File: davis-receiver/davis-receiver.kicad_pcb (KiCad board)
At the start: 4 copper layers, 127 x 88.9 mm, 150 parts, among them J1 Conn_Coaxial, J2 Wurth_74982104400, J3 JTAG, J4 UART, J5 SPI-BARO, J6 SPI-RF, Q1 FDC2512, SW1 MCU_RESET, T1 POE70P-33, U1 TM4C129ENCZADI3R, U2 CC1125RHBR, U3 FXPS7115D4, U4 TPS79930DDCR, U5 MB10S, U6 MB10S, U7 TPS23753A, U8 FOD817A3SD, U9 TLV431ACDBZR, X1 ECS-2520MV-400-AY-TR, Y1 LFXTAL071758CUTT

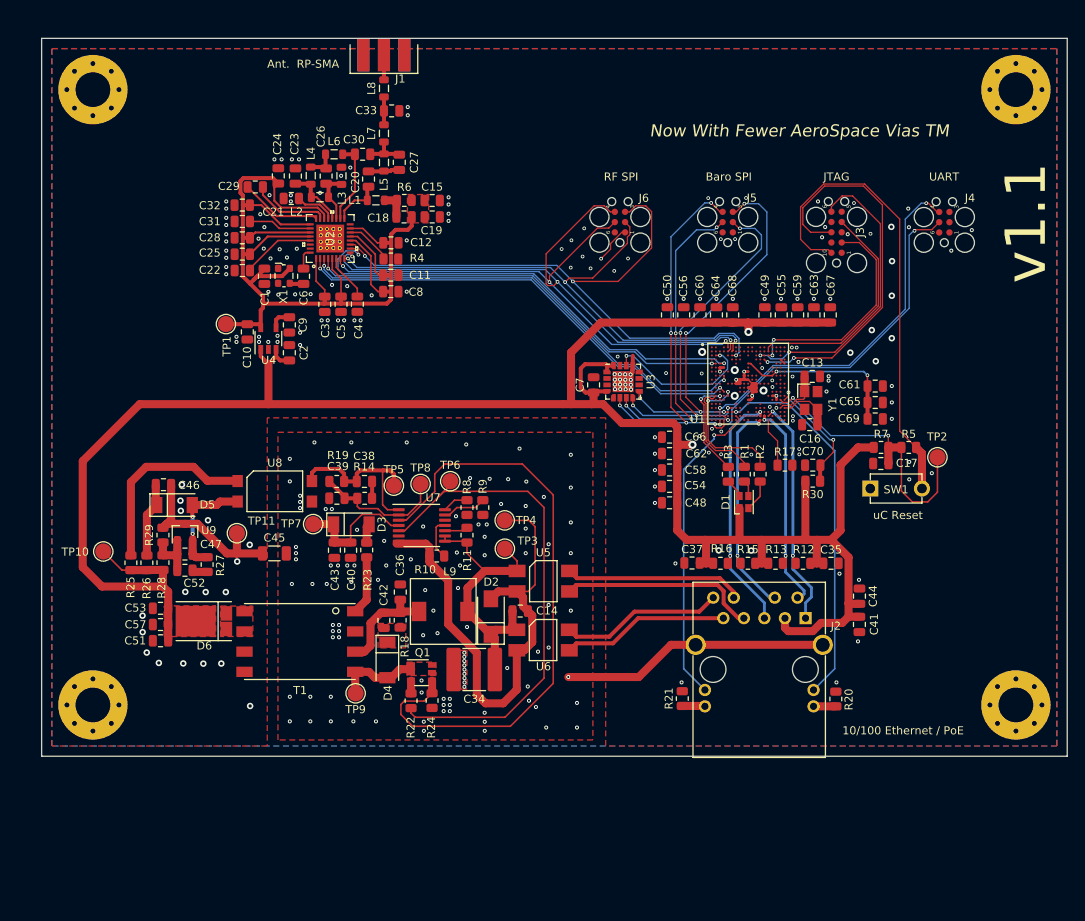
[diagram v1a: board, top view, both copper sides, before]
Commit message: Updates to DavisReceiver
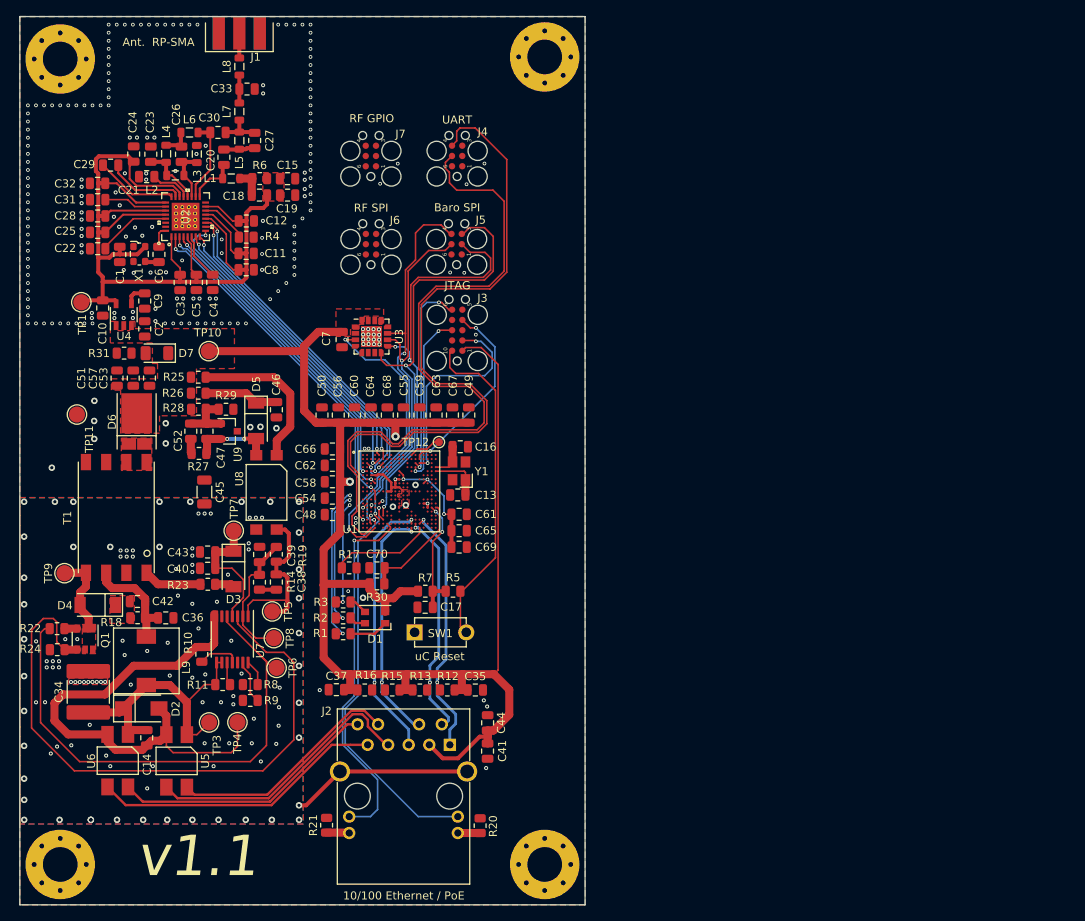
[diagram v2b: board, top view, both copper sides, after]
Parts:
- removed TP2: TestPoint, TestPoint:TestPoint_Pad_D2.0mm
- added D7: LED, LED_SMD:LED_1206_3216Metric, F.Cu at (39.0, 63.7)
- added J7: GPIO-RF, Custom:TC2030-IDC-FP, F.Cu at (65.5, 39.3)
- added R31: 100, Resistor_SMD:R_0805_2012Metric, F.Cu at (34.9, 63.7)
- added TP12: TestPoint, TestPoint:TestPoint_Pad_D1.0mm, F.Cu at (73.9, 74.7)
- C1, C2, C39, C49, C54, C55, C56, C58, C59, C60, C62, C63, C64, C66, C67, C68: value 0.1uF -> 100n
- C10: value 2.2uF -> 2u2
- C11, C12, C22, C25, C28, C3, C31, C32, C5, C8: value 0.047uF -> 47n
- C13, C16: value 22pF -> 8pF
- C18: value 33pF -> 33p
- C19, C47: value 100pF -> 100p
- C20: value 15pF -> 15p
- C21: value 10nF -> 10n
- C23, C26: value 3.3pF -> 3p3
- C24, C38: value 47nF -> 47n
- C27: value 1pF -> 1p
- C29: value 1.8nF -> 1n8
- C30: value 2.2pF -> 2p2
- C33: value 3pF -> 3p
- C34: value 22uF 63V -> 22u 63V
- C36: value 1uF 100V -> 1u 100V
- C4: value 220nF -> 220n
- C40: value 0.22uF -> 220n
- C42: value 10nF 100V -> 10n 100V
- C43: value 10uF -> 10u
- C46, C48: value 1uF -> 1u
- C50: value 01.uF -> 100n
- C51: value 47uf -> 47u
- C52: value 11900pF -> 11n9
- C53, C57: value 47uF -> 47u
- C6: value 22pF -> 22p
- C9: value 0.01uF -> 10n
- D1: footprint LED_SMD:LED_Cree-PLCC4_2x2mm_CW -> LED_SMD:LED_Cree-PLCC4_3.2x2.8mm_CCW
- L2: value 15nH -> 15n
- L3, L4, L6, L8: value 12nH -> 12n
- L5: value 7.5nH -> 7n5
- L7: value 18nH -> 18n
- L9: value 4.7uH SDR7030 -> 4u7 SDR7030
- R10: value 1.27K -> 1k27
- R11: value 24.9K -> 24k9
- R18: value 80K 0.1W -> 80k 0.1W
- R19: value 2K -> 2k
- R26: value 10K -> 10k
- R27: value 7.15K -> 7k15
- R28: value 41.2K -> 41k2
- R29: value 24.3K -> 24k3
- R4: value 56K -> 56k
- R8: value 59.0K -> 59k
- R9: value 80.6K -> 80k6
- moved H1 120.0 mm to (27.0, 127.0)
- moved J4 60.9 mm to (76.2, 39.3)
- moved H3 59.3 mm to (87.0, 127.0)
- moved C17 59.2 mm to (72.2, 95.2)
- moved SW1 59.2 mm to (74.1, 98.3)
- moved R5 59.2 mm to (75.6, 93.2), turned to 180 degrees
- moved R7 59.2 mm to (72.2, 93.2)
- moved H4 58.5 mm to (87.0, 27.0)
- moved C70 55.4 mm to (66.2, 90.3)
- moved R17 55.4 mm to (62.8, 90.3)
- moved R30 55.4 mm to (66.2, 92.3)
- moved U6 54.7 mm to (34.1, 114.1), turned to 180 degrees
- moved R2 54.6 mm to (62.0, 96.5), turned to 180 degrees
- moved C61 53.9 mm to (76.4, 83.6)
- moved C65 53.9 mm to (76.4, 85.7)
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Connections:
- net /BAR_CS renamed BAR_CS
- net /BAR_INT renamed BAR_INT
- net /BAR_MISO renamed BAR_MISO
- net /BAR_MOSI renamed BAR_MOSI
- net /BAR_SCLK renamed BAR_SCLK
- net /ETH_LED1 renamed ETH_LED1
- net /ETH_LED3 renamed ETH_LED3
- net /IND_B renamed IND_B
- net /JTAG_TCK renamed JTAG_TCK
- net /JTAG_TDI renamed JTAG_TDI
- net /JTAG_TDO renamed JTAG_TDO
- net /JTAG_TMS renamed JTAG_TMS
- net /PairOneNeg renamed PairOneNeg
- net /PairOnePos renamed PairOnePos
- net /PairTwoNeg renamed PairTwoNeg
- net /PairTwoPos renamed PairTwoPos
- net /RF_CS renamed RF_CS
- net /RF_GPIO0 renamed RF_GPIO0
- net /RF_GPIO2 renamed RF_GPIO2
- net /RF_GPIO3 renamed RF_GPIO3
- net /RF_MISO renamed RF_MISO
- net /RF_MOSI renamed RF_MOSI
- net /RF_RESET renamed RF_RESET
- net /RF_SCLK renamed RF_SCLK
- net /UART_RX renamed UART_RX
- net /UART_TX renamed UART_TX
- net Net-(C14-Pad2) renamed /VSS_POE
- D1 pad 1: +3V3 -> Net-(D1-Pad1)
- D1 pad 2: Net-(D1-Pad2) -> +3V3
- J3 pad 1: (no net) -> +3V3
- J3 pad 10: /JTAG_RESET -> ~JTAG_RESET~
- J3 pad 5: (no net) -> Net-(J3-Pad5)
- J3 pad 9: (no net) -> Net-(J3-Pad5)
- R1 pad 1: Net-(D1-Pad3) -> Net-(D1-Pad1)
- R1 pad 2: /IND_G -> IND_R
- R14 pad 1: Net-(C38-Pad1) -> Net-(C39-Pad1)
- R14 pad 2: Net-(C39-Pad1) -> Net-(C38-Pad2)
- R19 pad 1: Net-(C38-Pad2) -> Net-(C39-Pad1)
- R19 pad 2: Net-(C39-Pad1) -> Net-(C38-Pad1)
- R2 pad 2: /IND_R -> IND_G
- R3 pad 1: Net-(D1-Pad2) -> Net-(D1-Pad3)
- R5 pad 1: Net-(C17-Pad1) -> ~JTAG_RESET~
- R5 pad 2: /JTAG_RESET -> Net-(C17-Pad1)
- SW1 pad 2: /JTAG_RESET -> ~JTAG_RESET~
- TP5 pad 1: Net-(C38-Pad2) -> Net-(C38-Pad1)
- U1 pad A13: (no net) -> /DIVSCLK
- U1 pad D19: (no net) -> Net-(C16-Pad1)
- U1 pad E19: GND -> Net-(C13-Pad1)
- U1 pad N2: /IND_G -> IND_G
- U1 pad N5: /IND_R -> IND_R
- U1 pad T18: Net-(C13-Pad1) -> GND
- U1 pad T19: Net-(C16-Pad1) -> (no net)
- U7 pad 1: Net-(C38-Pad2) -> Net-(C38-Pad1)
- U8 pad 4: Net-(C38-Pad2) -> Net-(C38-Pad1)
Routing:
- net +3V3: track 323.6 -> 217.8 mm, vias 7 -> 5
- net /JTAG_RESET: track 58.3 -> 0.00 mm
- net UART_RX: track 45.7 -> 88.3 mm
- net UART_TX: track 44.2 -> 86.3 mm, vias 2 -> 0
- net ~JTAG_RESET~: track 0.00 -> 41.2 mm
- net RF_CS: track 76.1 -> 41.4 mm, vias 3 -> 2
- net RF_MISO: track 72.9 -> 40.1 mm, vias 3 -> 2
- net RF_SCLK: track 67.6 -> 37.0 mm, vias 3 -> 2
- net GND: track 30.2 -> 0.00 mm, vias 179 -> 221
- net RF_MOSI: track 65.2 -> 36.5 mm, vias 3 -> 2
- net JTAG_TDI: track 48.2 -> 21.2 mm
- net IND_R: track 0.00 -> 24.5 mm, vias 0 -> 3
- net IND_G: track 0.00 -> 21.2 mm, vias 0 -> 3
- net Net-(C17-Pad1): track 36.0 -> 15.0 mm
- net RF_GPIO0: track 59.1 -> 41.1 mm
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- added copper zone on B.Cu, net GND1
- added copper zone on In2.Cu, net GND1
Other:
- board size 127 x 88.9 mm -> 70 x 110 mm
- net class HV: clearance 0.127 -> 1
- board text added: "RF GPIO"
- board text removed: "Now With Fewer AeroSpace Vias TM"
